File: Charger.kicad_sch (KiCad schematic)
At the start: 59 parts, among them Q6 BSC0702LS, Q7 BSC0702LS, Q8 BSC0702LS, Q9 BSC0702LS, U27 BQ25756RRVR

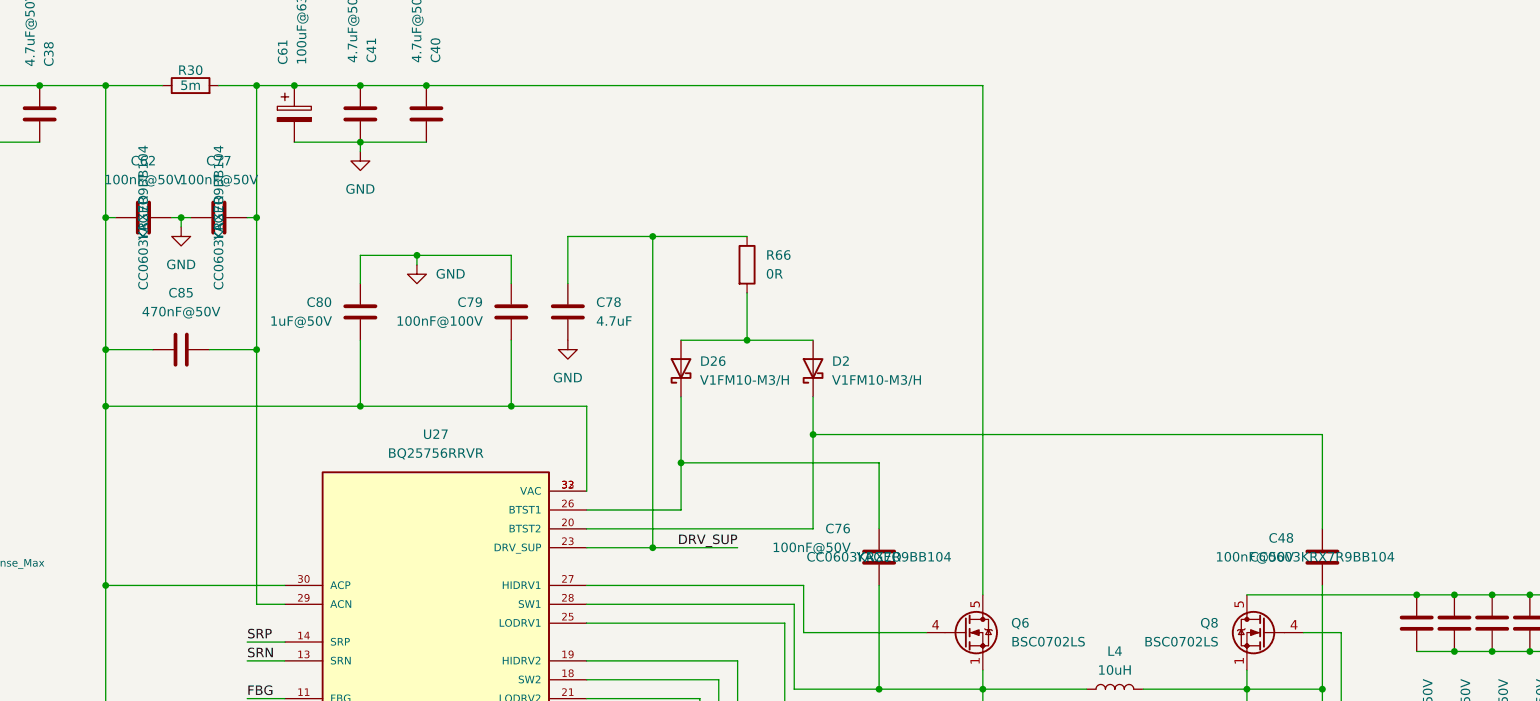
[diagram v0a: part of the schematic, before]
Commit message: Additional Infos
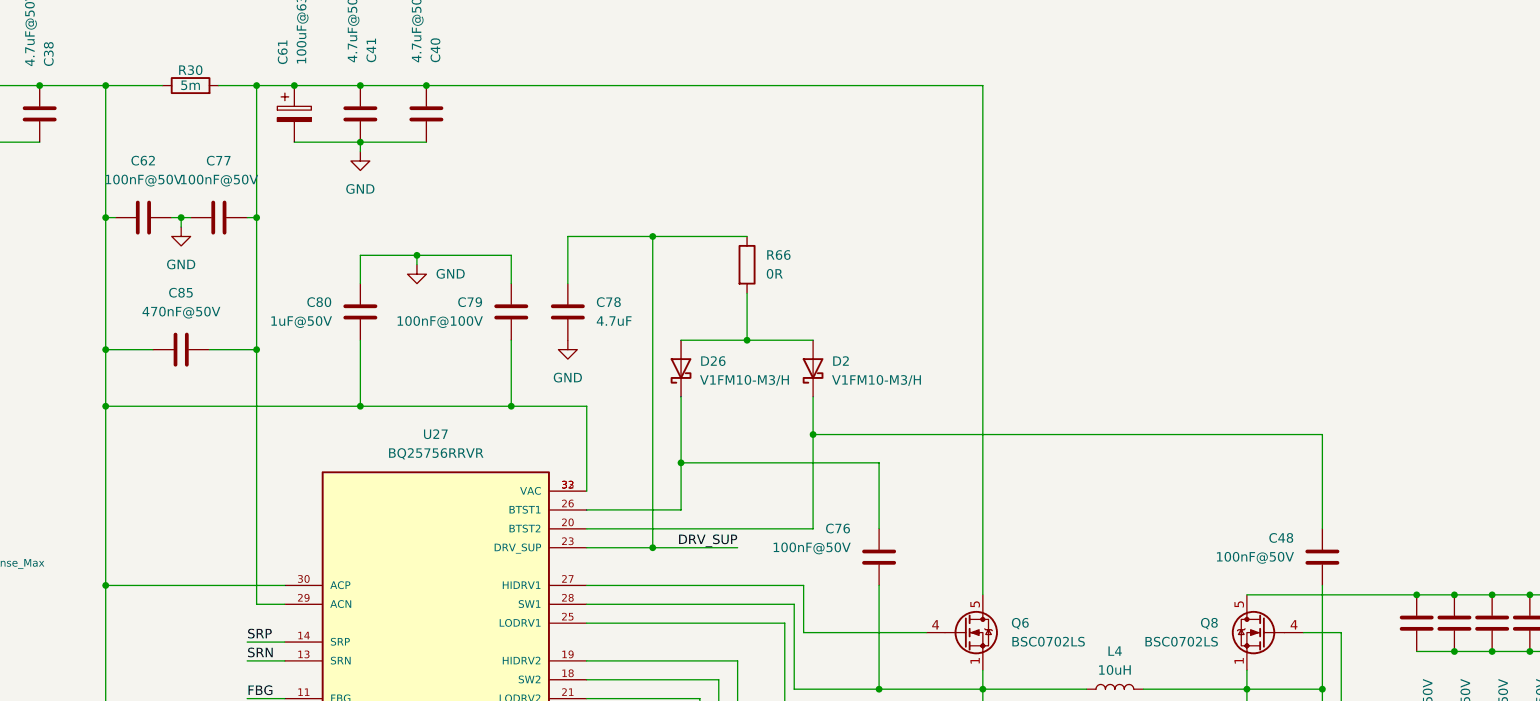
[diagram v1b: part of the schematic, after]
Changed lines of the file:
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@@
 					(size 1.27 1.27)
 				)
+				(hide yes)
 			)
 		)
@@
 					(size 1.27 1.27)
 				)
+				(hide yes)
 			)
 		)
@@
 					(size 1.27 1.27)
 				)
+				(hide yes)
 			)
 		)
@@
 					(size 1.27 1.27)
 				)
+				(hide yes)
 			)
 		)
@@
 					(size 1.27 1.27)
 				)
+				(hide yes)
 			)
 		)
@@
 					(size 1.27 1.27)
 				)
+				(hide yes)
 			)
 		)
@@
 					(size 1.27 1.27)
 				)
+				(hide yes)
 			)
 		)
